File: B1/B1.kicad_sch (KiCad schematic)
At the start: 1 part, among them U110 74HC04

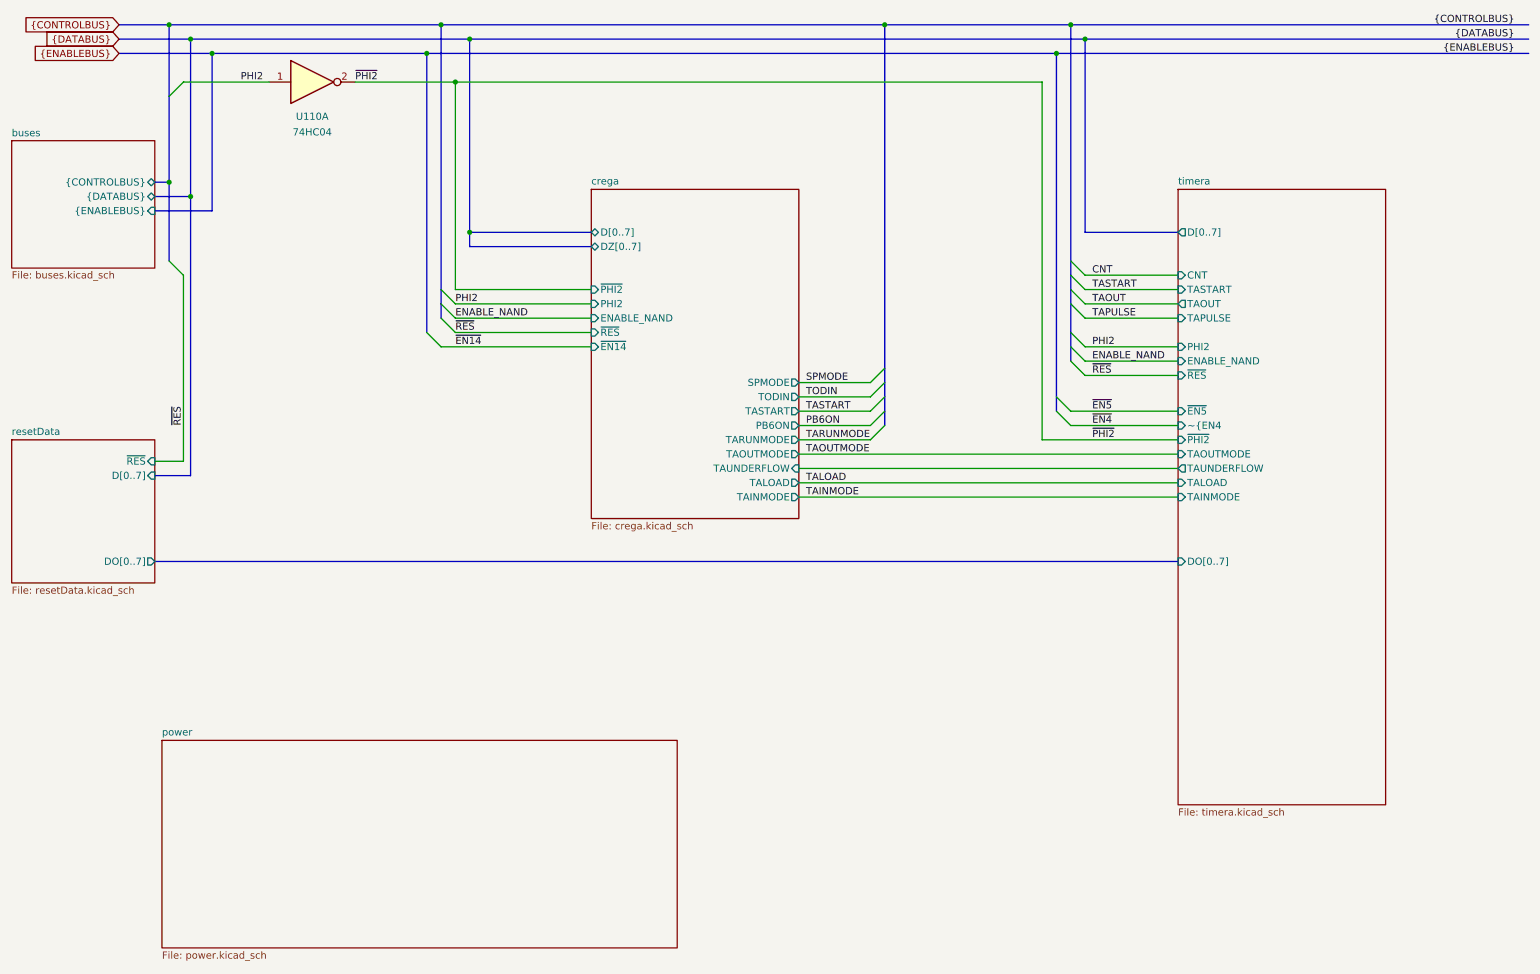
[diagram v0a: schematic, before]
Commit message: B2 almost ready
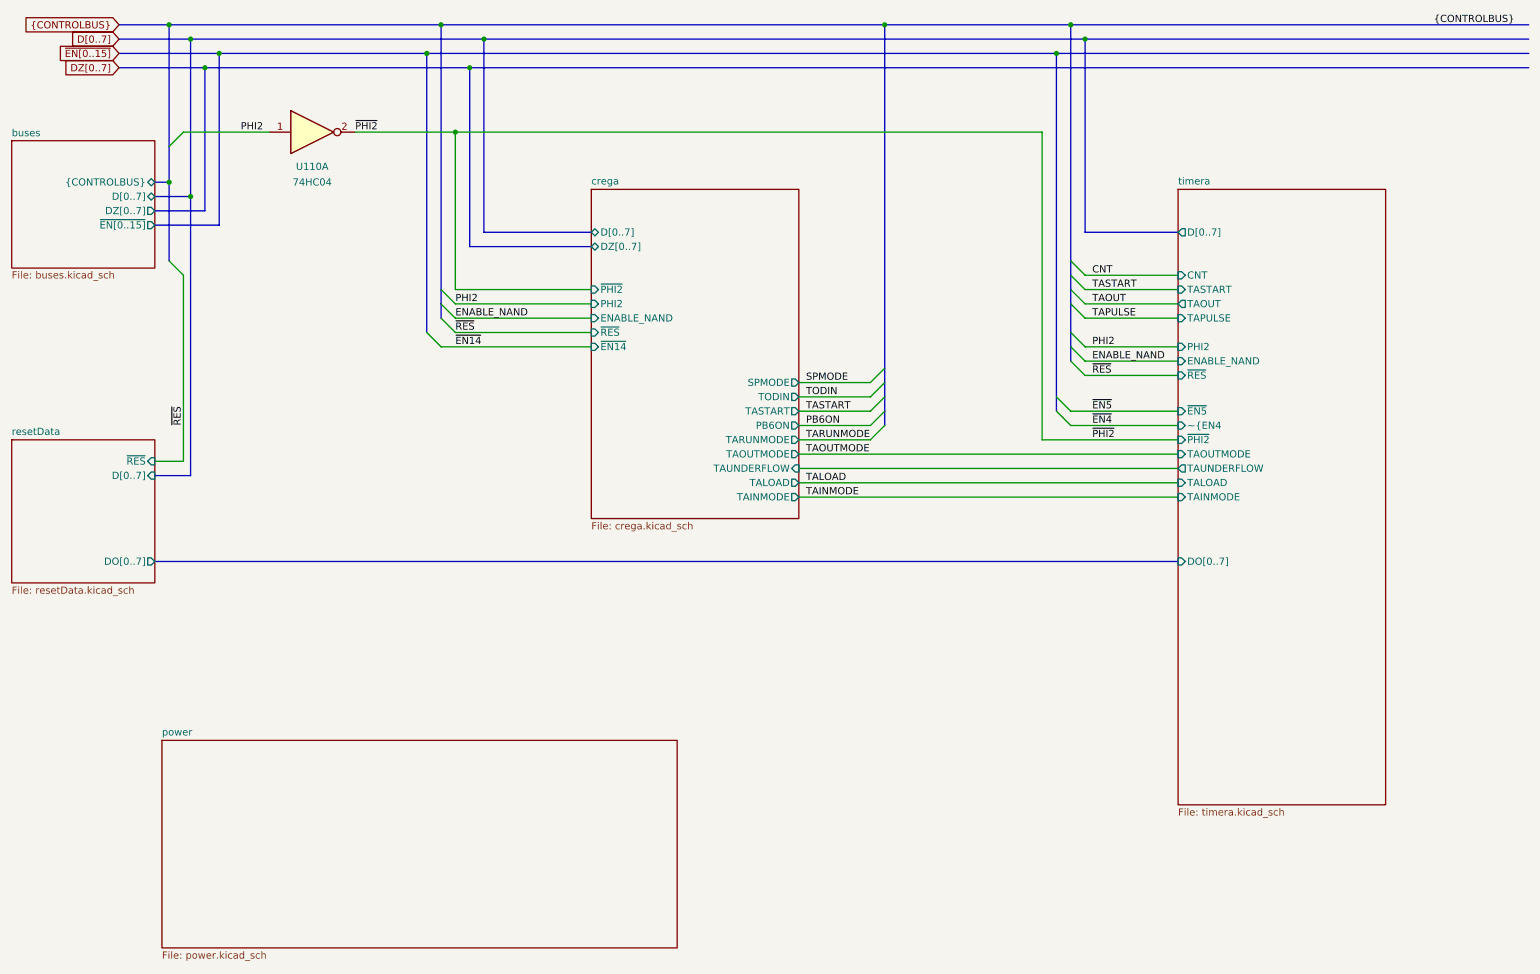
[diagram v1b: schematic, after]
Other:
- sheet buses ports: added DZ[0..7], D[0..7], ~{EN[0..15]}; removed {DATABUS}, {ENABLEBUS}
- moved on the sheet: U110A
